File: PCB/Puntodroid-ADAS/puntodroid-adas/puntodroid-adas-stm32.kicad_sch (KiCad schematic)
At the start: 6 parts, among them J1 USB_B, J2 BOOTLOADER, J3 SWD_INTERFACE, U1 STM32F446VETx

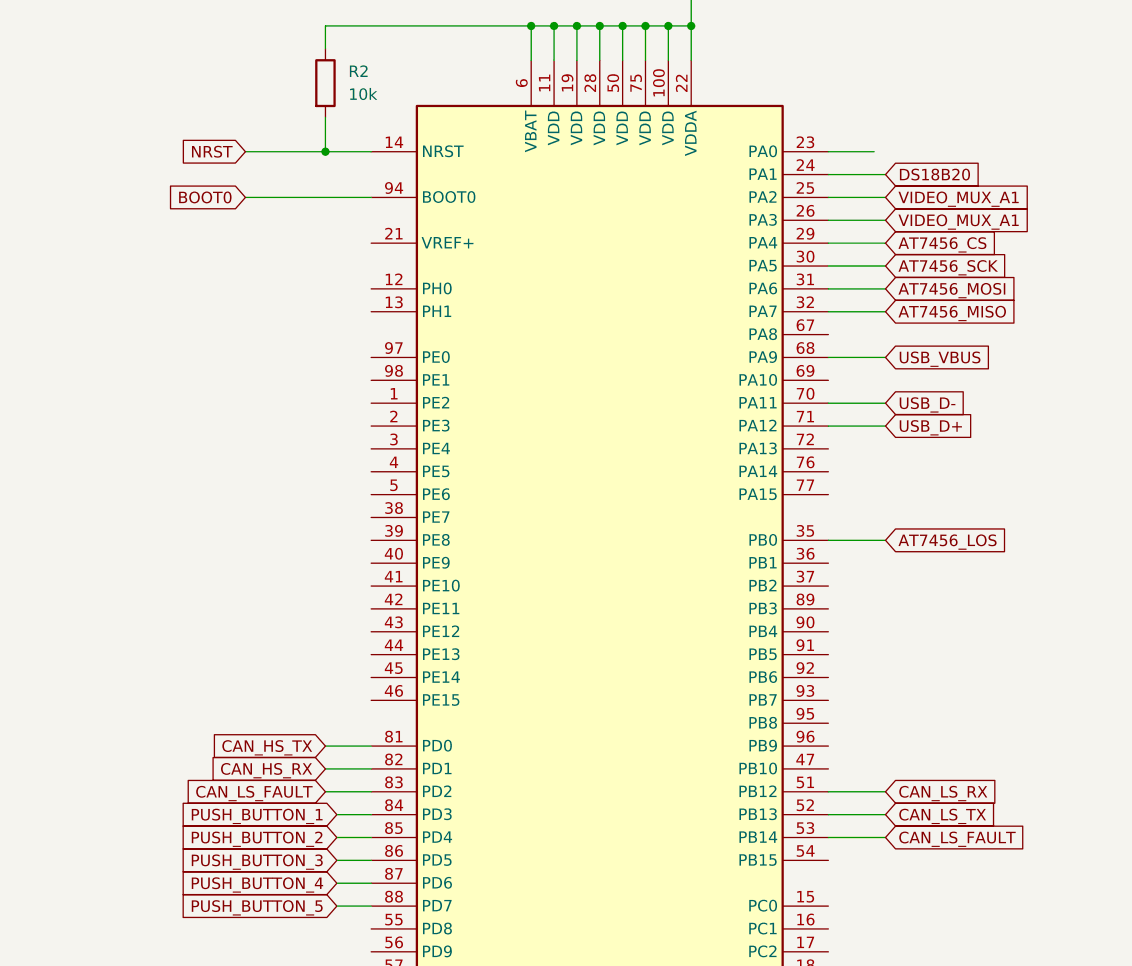
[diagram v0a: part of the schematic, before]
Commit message: UPDATE cube mx
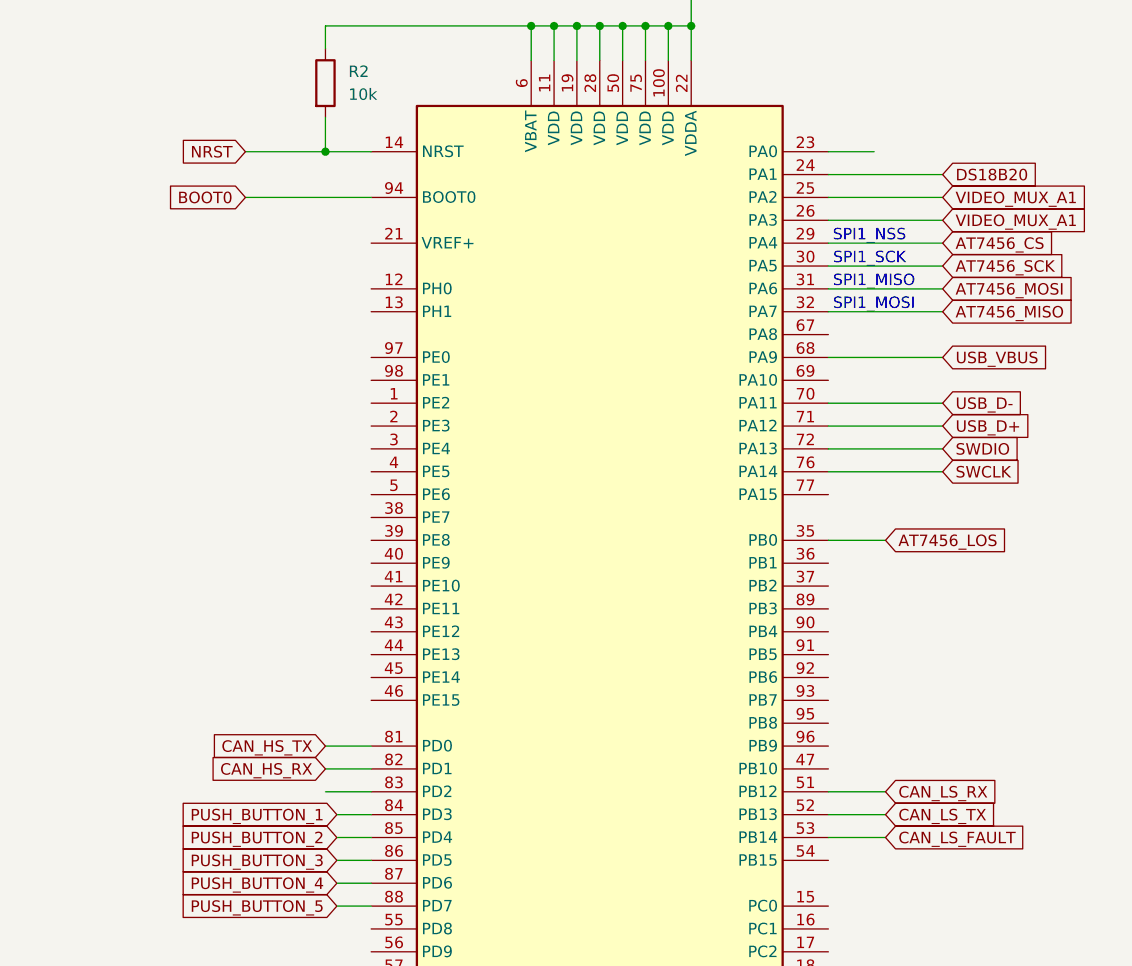
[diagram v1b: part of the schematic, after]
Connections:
- net CAN_LS_FAULT: no longer U1.83 (PD2)
- net SWCLK: now also U1.76 (PA14)
- net SWDIO: now also U1.72 (PA13)
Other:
- note added: "SPI1_MISO"
- note added: "SPI1_MOSI"
- note added: "SPI1_NSS"
- note added: "SPI1_SCK"

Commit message: update puntodroid
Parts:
- removed J3: SWD_INTERFACE, symbol Connector_Generic:Conn_01x06
- added C1, C2: 22p, symbol Device:C
- added C10, C12, C13, C5, C6, C7, C8, C9: 100n, symbol Device:C
- added C3, C4: 2u2, symbol Device:C_Polarized
- added J3: SWD PROGRAMMER, symbol Connector_Generic:Conn_01x05
- added R3: 5k6, symbol Device:R
- added R4, R5: 10k, symbol Device:R
- added U2: CM1293A, Package_TO_SOT_SMD:SOT-23-6, symbol Power_Protection:CDSOT236-0504C
- added Y1: 16MHz, symbol Device:Crystal
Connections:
- net +3V3: now also J2.1 (Pin_1), C10.2, C12.2, C13.2, C5.2, C6.2, C7.2, C8.2, C9.2, J3.2 (Pin_2), U2.5 (VP); no longer J2.6 (Pin_6)
- net BOOT0: now also J2.5 (Pin_5); no longer J2.2 (Pin_2)
- net BOOTLOADER_RX: now also J2.3 (Pin_3); no longer J2.4 (Pin_4)
- net BOOTLOADER_TX: now also J2.2 (Pin_2); no longer J2.5 (Pin_5)
- net CAN_LS_FAULT: now also U1.96 (PB9); no longer U1.53 (PB14)
- net CAN_LS_RX: now also U1.52 (PB13); no longer U1.51 (PB12)
- net CAN_LS_TX: now also U1.51 (PB12); no longer U1.52 (PB13)
- net DS18B20: now also U1.83 (PD2); no longer U1.24 (PA1)
- net GNDD: now also J2.6 (Pin_6), C1.1, C10.1, C12.1, C13.1, C2.1, C3.2, C4.2, C5.1, C6.1, C7.1, C8.1, C9.1, J3.3 (Pin_3), R4.2, R5.2, U2.2 (VN); no longer J2.1 (Pin_1)
- net NRST: now also J2.4 (Pin_4), J3.1 (Pin_1); no longer J2.3 (Pin_3)
- net PUSH_BUTTON_1: now also U1.5 (PE6); no longer U1.84 (PD3)
- net PUSH_BUTTON_2: now also U1.15 (PC0); no longer U1.85 (PD4)
- net PUSH_BUTTON_3: now also U1.16 (PC1); no longer U1.86 (PD5)
- net PUSH_BUTTON_4: now also U1.17 (PC2); no longer U1.87 (PD6)
- net PUSH_BUTTON_5: now also U1.18 (PC3); no longer U1.88 (PD7)
- net SWCLK: now also J3.5 (Pin_5)
- net SWDIO: now also J3.4 (Pin_4)
- net USB_D+: now also U2.4 (IO3), U2.6 (IO4)
- net USB_D-: now also U2.1 (IO1), U2.3 (IO2)
- net USB_VBUS: now also R3.2, R4.1; no longer J1.1 (VBUS)
- net VIDEO_MUX_A1: now also U1.36 (PB1); no longer U1.25 (PA2), U1.26 (PA3)
- net PE2_UNUSED: now reaches U1.1 (PE2)
- net at U1.12 (PH0): now also C1.2, Y1.2
- net at U1.13 (PH1): now also C2.2, Y1.1
- net PE3_UNUSED: now reaches U1.2 (PE3)
- net ADC_VBATT_12V: now reaches U1.23 (PA0)
- net PE4_UNUSED: now reaches U1.3 (PE4)
- net at U1.37 (PB2): now also R5.1
- net VIDEO_MUX_A2: now reaches U1.38 (PE7)
- net PE8_UNUSED: now reaches U1.39 (PE8)
- net PUSH_BUTTON_0: now reaches U1.4 (PE5)
- net PE9_UNUSED: now reaches U1.40 (PE9)
- net P10_UNUSED: now reaches U1.41 (PE10)
- net PE11_UNUSED: now reaches U1.42 (PE11)
- net PE12_UNUSED: now reaches U1.43 (PE12)
- net PE13_UNUSED: now reaches U1.44 (PE13)
- net PE14_UNUSED: now reaches U1.45 (PE14)
- net RFM69_CS: now reaches U1.46 (PE15)
- net RFM69_SCK: now reaches U1.47 (PB10)
- net at U1.48 (VCAP_1): now also C4.1
- net RFM69_MISO: now reaches U1.54 (PB15)
- net PD8_UNUSED: now reaches U1.55 (PD8)
- net PD9_UNUSED: now reaches U1.56 (PD9)
- net PD10_UNUSED: now reaches U1.57 (PD10)
- net PD11_UNUSED: now reaches U1.58 (PD11)
- net PD12_UNUSED: now reaches U1.59 (PD12)
- net PD13_UNUSED: now reaches U1.60 (PD13)
- net PD14_UNUSED: now reaches U1.61 (PD14)
- net PD15_UNUSED: now reaches U1.62 (PD15)
- net PC6_UNUSED: now reaches U1.63 (PC6)
- net PC7_UNUSED: now reaches U1.64 (PC7)
- net PC8_UNUSED: now reaches U1.65 (PC8)
- net PC9_UNUSED: now reaches U1.66 (PC9)
- net PA8_UNUSED: now reaches U1.67 (PA8)
- net PA10_UNUSED: now reaches U1.69 (PA10)
- net PC13_UNUSED: now reaches U1.7 (PC13)
- net at U1.73 (VCAP_2): now also C3.1
- net BOOTLOADER_DEBUG_RX: now reaches U1.78 (PC10)
- net BOOTLOADER_DEBUG_TX: now reaches U1.79 (PC11)
- net PC14_UNUSED: now reaches U1.8 (PC14)
- net PC12_UNUSED: now reaches U1.80 (PC12)
- net PB3_UNUSED: now reaches U1.89 (PB3)
- net PC15_UNUSED: now reaches U1.9 (PC15)
- net PB4_UNUSED: now reaches U1.90 (PB4)
- net PB5_UNUSED: now reaches U1.91 (PB5)
- net PB6_UNUSED: now reaches U1.92 (PB6)
- net PB7_UNUSED: now reaches U1.93 (PB7)
- net PB8_UNUSED: now reaches U1.95 (PB8)
- net PE0_UNUSED: now reaches U1.97 (PE0)
- net PE1_UNUSED: now reaches U1.98 (PE1)
- new net: J1.1 (VBUS), R3.1
- new net ADC_5V: U1.24 (PA1)
- new net BUZZER_OUT: U1.84 (PD3)
- new net LPGTECH_RX: U1.25 (PA2)
- new net LPGTECH_TX: U1.26 (PA3)
- new net PD5_UNUSED: U1.86 (PD5)
- new net PD6_UNUSED: U1.87 (PD6)
- new net PD7_UNUSED: U1.88 (PD7)
- new net REVERSE_SIGNAL: U1.85 (PD4)
- new net RFM69_MOSI: U1.53 (PB14)
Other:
- note added: "16MHz CRYSTAL"
- note added: "ADC_IN0"
- note added: "ADC_IN1"
- note added: "BOOT1 configuration"
- note added: "BOOTLOADER DEBUG UART"
- note added: "CAN2_RX"
- note added: "CAN2_TX"
- note added: "RCC_OSC_IN"
- note added: "RCC_OSC_OUT"
- note added: "SPI2_MISO"
- note added: "SPI2_MOSI"
- note added: "SPI2_SCK"
- note added: "SWD PROGRAMMING"
- note added: "USART2_RX"
- note added: "USART2_TX"
- note added: "USART3_RX"
- note added: "USART3_TX"
- note added: "USB SOCKET"
- moved on the sheet: J1, J2, R1
